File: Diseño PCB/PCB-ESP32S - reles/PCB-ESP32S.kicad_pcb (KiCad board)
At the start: 2 copper layers, 109.2 x 83.8 mm, 40 parts, among them J1 Screw_Terminal_01x03, J3 Screw_Terminal_01x03, J7 Screw_Terminal_01x03, J8 Screw_Terminal_01x02, K1 SRD-05VDC-SL-C, K2 SRD-05VDC-SL-C, Q1 MMBT2222A, Q2 MMBT2222A, Q3 TIP42C, SW1 SW_DIP_x01, SW2 SW_DIP_x01, U1 ESP-32S, U3 PC817, U4 PC817, U5 LM7805_TO220, U6 LM1117-3.3

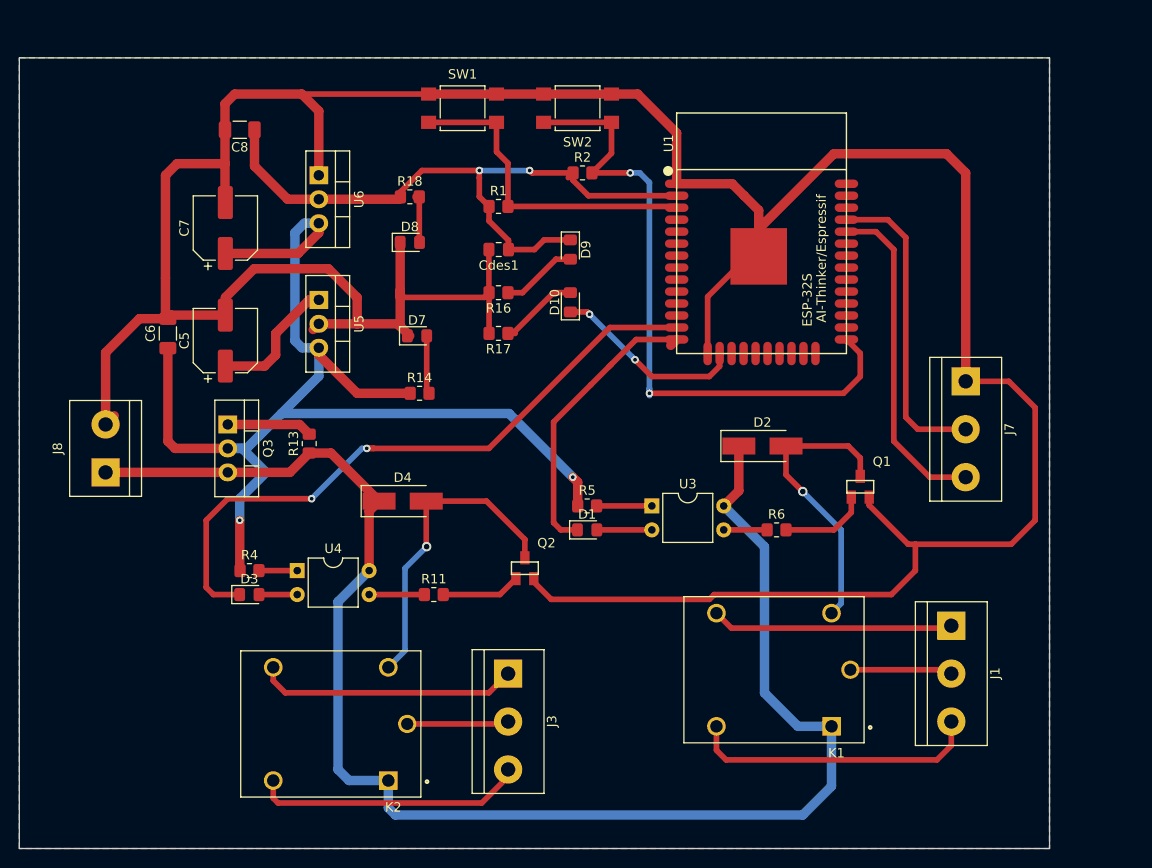
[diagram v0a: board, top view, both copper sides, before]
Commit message: PCB reles
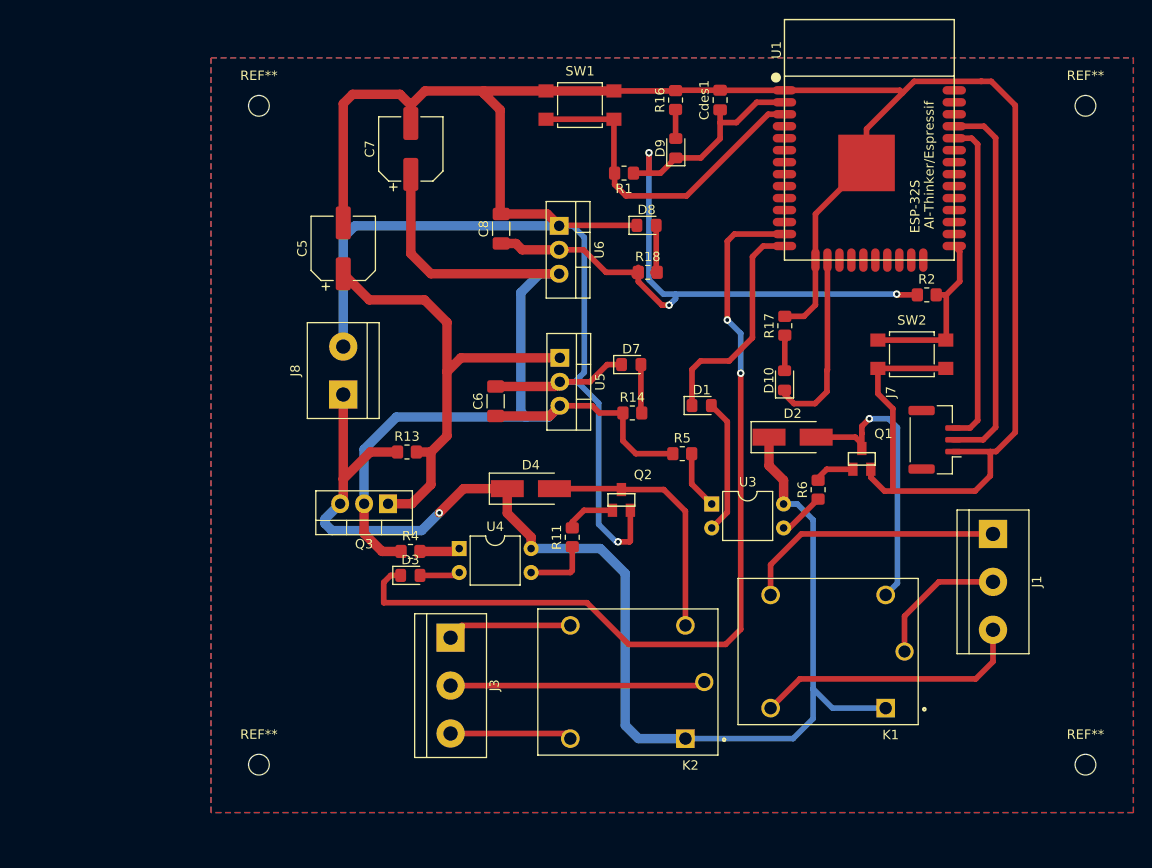
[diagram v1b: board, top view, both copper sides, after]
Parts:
- added REF**: MountingHole_2.2mm_M2, MountingHole:MountingHole_2.2mm_M2, F.Cu at (285.8, 91.4)
- added REF**: MountingHole_2.2mm_M2, MountingHole:MountingHole_2.2mm_M2, F.Cu at (198.1, 91.4)
- added REF**: MountingHole_2.2mm_M2, MountingHole:MountingHole_2.2mm_M2, F.Cu at (198.1, 21.6)
- added REF**: MountingHole_2.2mm_M2, MountingHole:MountingHole_2.2mm_M2, F.Cu at (285.8, 21.6)
- J7: footprint TerminalBlock:TerminalBlock_bornier-3_P5.08mm -> Connector_JST:JST_GH_BM03B-GHS-TBT_1x03-1MP_P1.25mm_Vertical
- moved SW2 44.0 mm to (267.3, 47.9), turned to 0 degrees
- moved R2 38.7 mm to (268.9, 41.6)
- moved C6 35.5 mm to (223.2, 52.9)
- moved K2 31.8 mm to (237.2, 82.7)
- moved R17 30.4 mm to (253.9, 44.9), turned to 90 degrees
- moved C8 29.6 mm to (223.8, 34.6), turned to 90 degrees
- moved Cdes1 28.3 mm to (247.0, 21.0), turned to 90 degrees
- moved R16 27.7 mm to (242.3, 21.0), turned to 90 degrees
- moved J8 26.5 mm to (207.1, 52.2)
- moved R18 26.5 mm to (239.3, 39.2)
- moved U5 26.3 mm to (230.0, 48.3)
- moved U6 26.0 mm to (229.9, 34.3)
- moved D8 25.2 mm to (239.2, 34.3)
- moved D10 24.2 mm to (253.8, 50.7)
- moved D7 22.9 mm to (237.6, 49.0)
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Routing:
- net Net-(R2-Pad2): track 70.7 -> 19.6 mm, vias 2 -> 0
- net Net-(C5-Pad1): track 23.2 -> 50.5 mm
- net +5V: track 127.2 -> 102.7 mm, vias 2 -> 0
- net IO14: track 69.8 -> 92.7 mm
- net +12V: track 163.1 -> 140.4 mm, vias 0 -> 1
- net GND: track 345.2 -> 325.0 mm, vias 0 -> 2
- net +3V3: track 71.2 -> 90.3 mm, vias 2 -> 3
- net /ModulosReles/C: track 10.8 -> 27.4 mm
- net /ModulosReles/NC: track 28.9 -> 13.7 mm
- net /ModulosReles/NO: track 29.1 -> 14.8 mm
- net Net-(D1-Pad2): track 5.83 -> 14.4 mm
- net Net-(J7-Pad2): track 33.0 -> 40.6 mm
- net IO12: track 31.4 -> 24.1 mm
- net Net-(D4-Pad2): track 33.4 -> 27.0 mm, vias 1 -> 0
- net Net-(D9-Pad2): track 8.09 -> 3.09 mm
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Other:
- board outline removed
